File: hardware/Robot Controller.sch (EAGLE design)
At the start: 18 parts

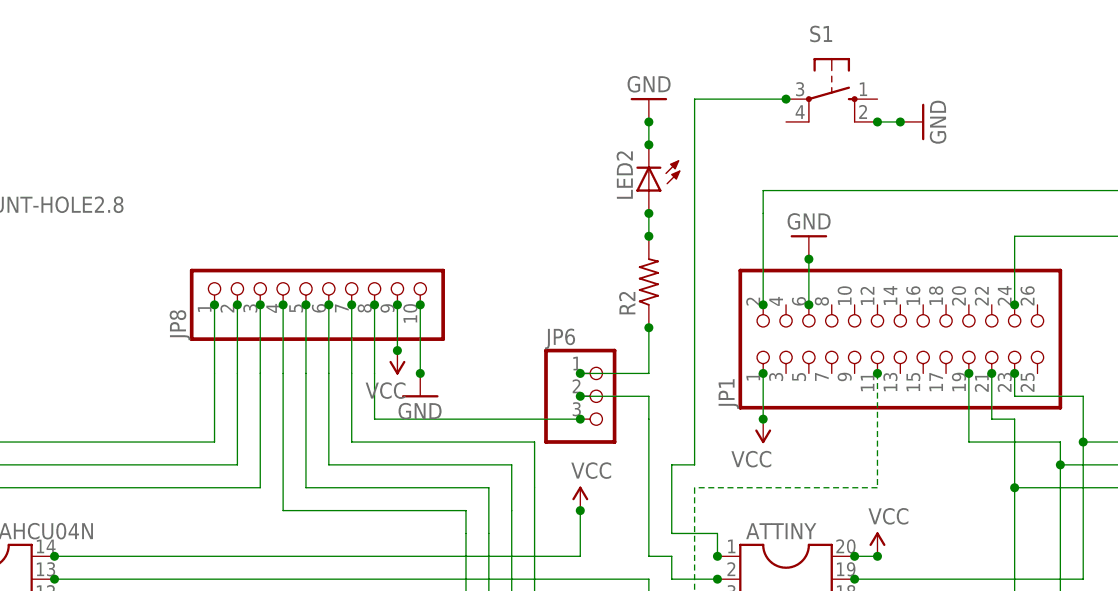
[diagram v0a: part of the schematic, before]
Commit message: tighten up PCB
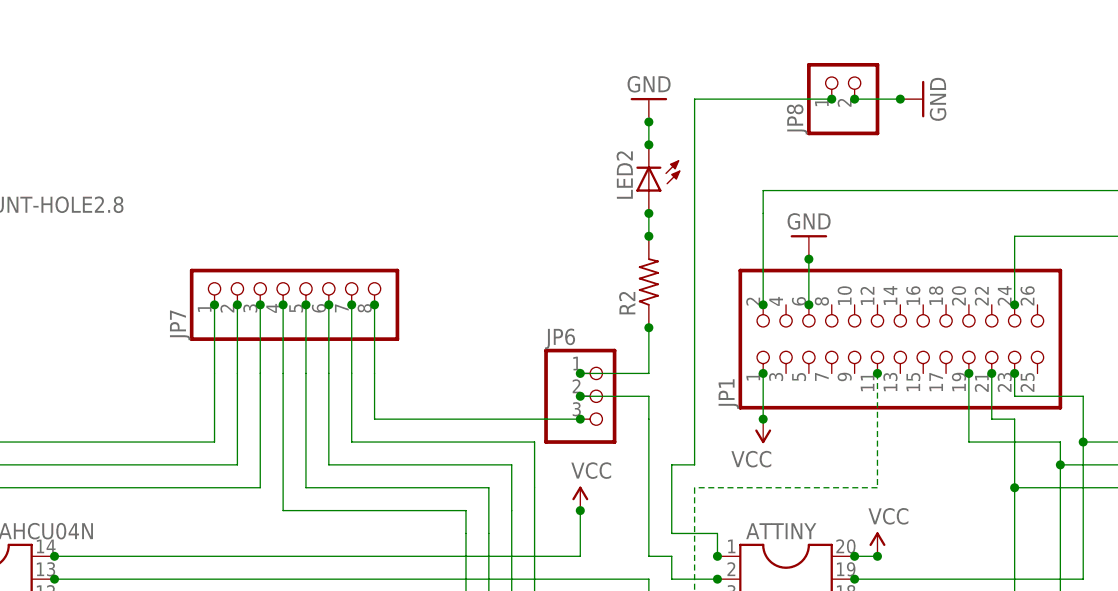
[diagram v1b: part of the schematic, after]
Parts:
- removed S1: (no value), switch-omron:10-XX
- added JP7: (no value), pinhead:PINHD-1X8
- JP8: device pinhead:PINHD-1X10 -> pinhead:PINHD-1X2
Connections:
- net GND: now also JP8.2; no longer JP8.10, S1.S1
- net N$23: now also JP7.8; no longer JP8.8
- net N$24: now also JP7.7; no longer JP8.7
- net N$25: now also JP7.6; no longer JP8.6
- net N$26: now also JP7.5; no longer JP8.5
- net N$27: now also JP7.4; no longer JP8.4
- net N$28: now also JP7.1; no longer JP8.1
- net N$29: now also JP7.2; no longer JP8.2
- net N$30: now also JP7.3; no longer JP8.3
- net N$31: now also JP8.1; no longer S1.P
- net VCC: no longer JP8.9
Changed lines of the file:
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@@
 <part name="SUPPLY4" library="SparkFun-Aesthetics" deviceset="VCC" device=""/>
 <part name="JP6" library="pinhead" deviceset="PINHD-1X3" device=""/>
-<part name="JP8" library="pinhead" deviceset="PINHD-1X10" device=""/>
-<part name="SUPPLY5" library="SparkFun-Aesthetics" deviceset="VCC" device=""/>
-<part name="GND11" library="SparkFun-Aesthetics" deviceset="GND" device=""/>
-<part name="S1" library="switch-omron" deviceset="10-XX" device=""/>
 <part name="GND12" library="SparkFun-Aesthetics" deviceset="GND" device=""/>
+<part name="JP7" library="pinhead" deviceset="PINHD-1X8" device=""/>
+<part name="JP8" library="pinhead" deviceset="PINHD-1X2" device=""/>
 </parts>
 <sheets>
@@
 <instance part="SUPPLY4" gate="1" x="121.92" y="86.36" rot="R180"/>
 <instance part="JP6" gate="A" x="38.1" y="91.44"/>
-<instance part="JP8" gate="A" x="5.08" y="104.14" rot="R90"/>
-<instance part="SUPPLY5" gate="1" x="15.24" y="96.52" rot="R180"/>
-<instance part="GND11" gate="1" x="17.78" y="91.44"/>
-<instance part="S1" gate="1" x="63.5" y="124.46" rot="R270"/>
-<instance part="GND12" gate="1" x="73.66" y="121.92" rot="R90"/>
+<instance part="GND12" gate="1" x="73.66" y="124.46" rot="R90"/>
+<instance part="JP7" gate="A" x="5.08" y="104.14" rot="R90"/>
+<instance part="JP8" gate="G$1" x="66.04" y="127" rot="R90"/>
 </instances>
 <busses>
@@
 </segment>
 <segment>
-<pinref part="JP8" gate="A" pin="10"/>
-<pinref part="GND11" gate="1" pin="GND"/>
-<wire x1="17.78" y1="101.6" x2="17.78" y2="93.98" width="0.1524" layer="91"/>
-<junction x="17.78" y="101.6"/>
-<junction x="17.78" y="93.98"/>
-</segment>
-<segment>
-<pinref part="S1" gate="1" pin="S1"/>
 <pinref part="GND12" gate="1" pin="GND"/>
-<wire x1="68.58" y1="121.92" x2="71.12" y2="121.92" width="0.1524" layer="91"/>
-<junction x="68.58" y="121.92"/>
-<junction x="71.12" y="121.92"/>
+<wire x1="66.04" y1="124.46" x2="71.12" y2="124.46" width="0.1524" layer="91"/>
+<junction x="71.12" y="124.46"/>
+<pinref part="JP8" gate="G$1" pin="2"/>
+<junction x="66.04" y="124.46"/>
 </segment>
 </net>
@@
 <junction x="121.92" y="86.36"/>
 <junction x="119.38" y="96.52"/>
-</segment>
-<segment>
-<pinref part="JP8" gate="A" pin="9"/>
-<pinref part="SUPPLY5" gate="1" pin="VCC"/>
-<wire x1="15.24" y1="101.6" x2="15.24" y2="96.52" width="0.1524" layer="91"/>
-<junction x="15.24" y="96.52"/>
-<junction x="15.24" y="101.6"/>
 </segment>
 </net>
@@
 <wire x1="12.7" y1="88.9" x2="35.56" y2="88.9" width="0.1524" layer="91"/>
 <junction x="35.56" y="88.9"/>
-<pinref part="JP8" gate="A" pin="8"/>
 <wire x1="12.7" y1="93.98" x2="12.7" y2="101.6" width="0.1524" layer="91"/>
+<pinref part="JP7" gate="A" pin="8"/>
 <junction x="12.7" y="101.6"/>
 </segment>
@@
 <wire x1="10.16" y1="86.36" x2="10.16" y2="93.98" width="0.1524" layer="91"/>
 <junction x="50.8" y="60.96"/>
-<pinref part="JP8" gate="A" pin="7"/>
 <wire x1="10.16" y1="93.98" x2="10.16" y2="101.6" width="0.1524" layer="91"/>
+<pinref part="JP7" gate="A" pin="7"/>
 <junction x="10.16" y="101.6"/>
 </segment>
@@
 <wire x1="7.62" y1="83.82" x2="7.62" y2="93.98" width="0.1524" layer="91"/>
 <junction x="50.8" y="58.42"/>
-<pinref part="JP8" gate="A" pin="6"/>
 <wire x1="7.62" y1="93.98" x2="7.62" y2="101.6" width="0.1524" layer="91"/>
+<pinref part="JP7" gate="A" pin="6"/>
 <junction x="7.62" y="101.6"/>
 </segment>
@@
 <wire x1="5.08" y1="81.28" x2="5.08" y2="93.98" width="0.1524" layer="91"/>
 <junction x="50.8" y="55.88"/>
-<pinref part="JP8" gate="A" pin="5"/>
 <wire x1="5.08" y1="93.98" x2="5.08" y2="101.6" width="0.1524" layer="91"/>
+<pinref part="JP7" gate="A" pin="5"/>
 <junction x="5.08" y="101.6"/>
 </segment>
@@
 <wire x1="2.54" y1="78.74" x2="2.54" y2="93.98" width="0.1524" layer="91"/>
 <junction x="50.8" y="53.34"/>
-<pinref part="JP8" gate="A" pin="4"/>
 <wire x1="2.54" y1="93.98" x2="2.54" y2="101.6" width="0.1524" layer="91"/>
+<pinref part="JP7" gate="A" pin="4"/>
 <junction x="2.54" y="101.6"/>
 </segment>
@@
 <wire x1="-5.08" y1="86.36" x2="-5.08" y2="93.98" width="0.1524" layer="91"/>
 <junction x="66.04" y="55.88"/>
-<pinref part="JP8" gate="A" pin="1"/>
 <wire x1="-5.08" y1="93.98" x2="-5.08" y2="101.6" width="0.1524" layer="91"/>
+<pinref part="JP7" gate="A" pin="1"/>
 <junction x="-5.08" y="101.6"/>
 </segment>
@@
 <wire x1="-2.54" y1="83.82" x2="-2.54" y2="93.98" width="0.1524" layer="91"/>
 <junction x="66.04" y="53.34"/>
-<pinref part="JP8" gate="A" pin="2"/>
 <wire x1="-2.54" y1="93.98" x2="-2.54" y2="101.6" width="0.1524" layer="91"/>
+<pinref part="JP7" gate="A" pin="2"/>
 <junction x="-2.54" y="101.6"/>
 </segment>
@@
 <wire x1="0" y1="81.28" x2="0" y2="93.98" width="0.1524" layer="91"/>
 <junction x="66.04" y="50.8"/>
-<pinref part="JP8" gate="A" pin="3"/>
 <wire x1="0" y1="93.98" x2="0" y2="101.6" width="0.1524" layer="91"/>
+<pinref part="JP7" gate="A" pin="3"/>
 <junction x="0" y="101.6"/>
 </segment>
@@
 <wire x1="45.72" y1="83.82" x2="48.26" y2="83.82" width="0.1524" layer="91"/>
 <wire x1="48.26" y1="83.82" x2="48.26" y2="124.46" width="0.1524" layer="91"/>
-<pinref part="S1" gate="1" pin="P"/>
-<wire x1="48.26" y1="124.46" x2="58.42" y2="124.46" width="0.1524" layer="91"/>
+<wire x1="48.26" y1="124.46" x2="63.5" y2="124.46" width="0.1524" layer="91"/>
 <junction x="50.8" y="73.66"/>
-<junction x="58.42" y="124.46"/>
-</segment>
-</net>
+<pinref part="JP8" gate="G$1" pin="1"/>
+<junction x="63.5" y="124.46"/>
+</segment>
+</net>
